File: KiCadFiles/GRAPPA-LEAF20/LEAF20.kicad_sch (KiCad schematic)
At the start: 48 parts

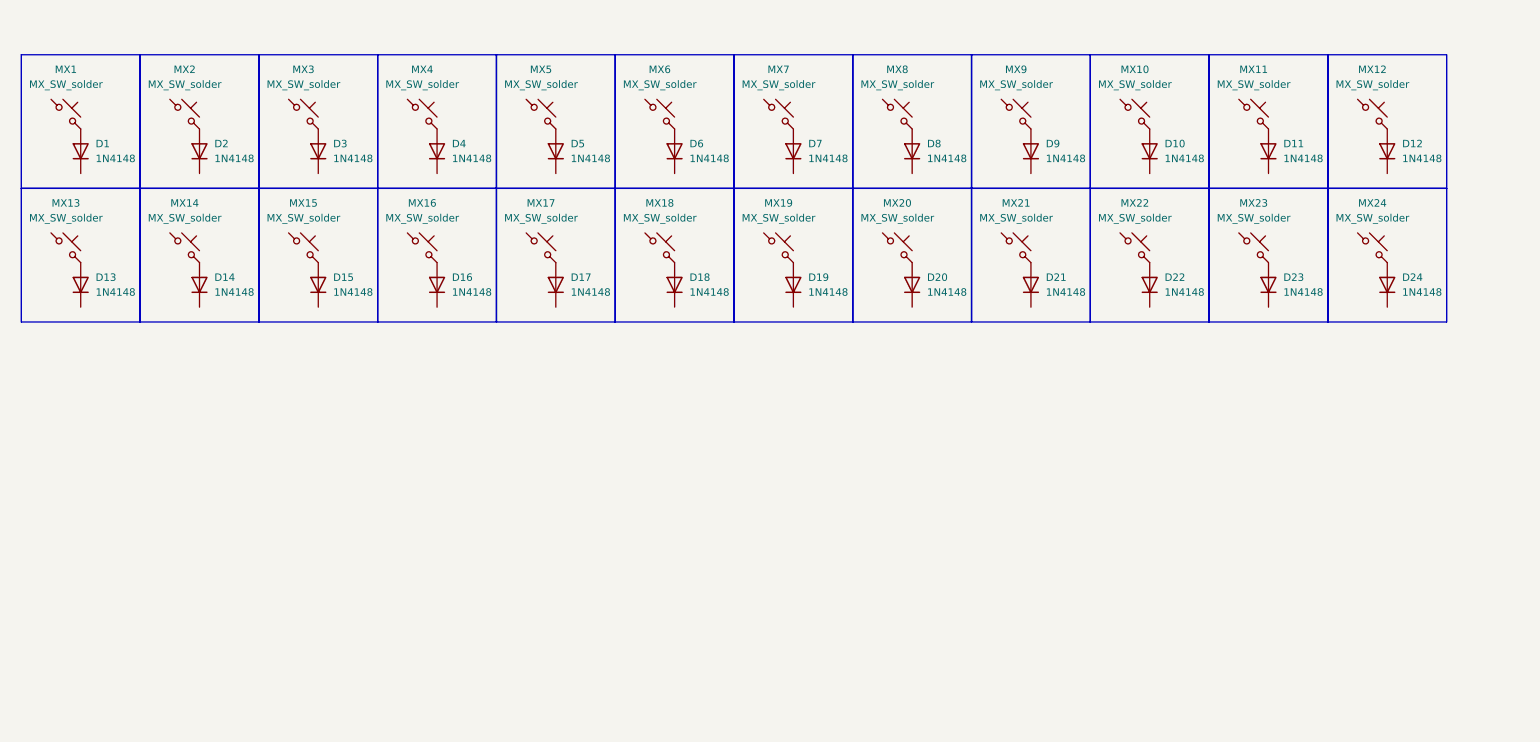
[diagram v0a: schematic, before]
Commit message: Refactor code structure for improved readability and maintainability
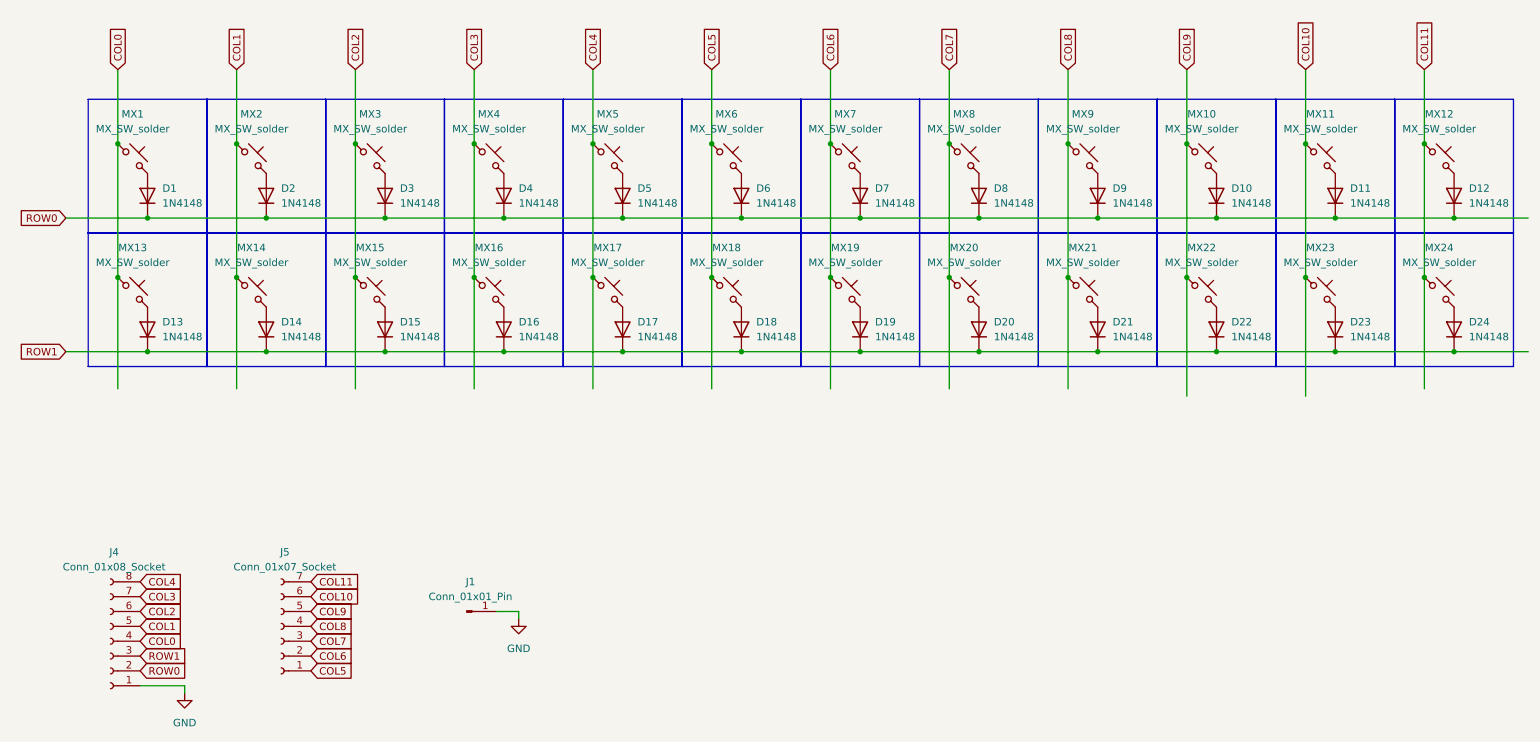
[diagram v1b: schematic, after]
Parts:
- added J1: Conn_01x01_Pin, Connector_Wire:SolderWire-0.75sqmm_1x01_D1.25mm_OD2.3mm, symbol Connector:Conn_01x01_Pin
- added J4: Conn_01x08_Socket, Connector_JST:JST_SH_SM08B-SRSS-TB_1x08-1MP_P1.00mm_Horizontal, symbol Connector:Conn_01x08_Socket
- added J5: Conn_01x07_Socket, Connector_JST:JST_SH_SM07B-SRSS-TB_1x07-1MP_P1.00mm_Horizontal, symbol Connector:Conn_01x07_Socket
- D1, D10, D11, D12, D13, D14, D15, D16, D17, D18, D19, D2, D20, D21, D22, D23, D24, D3, D4, D5, D6, D7, D8, D9: footprint Diode_SMD:D_SOD-323_HandSoldering -> My-Fi Footprints:D_SOD-123-g
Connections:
- net COL3: now reaches MX16.1
- net COL3: now also MX4.1, J4.7 (Pin_7)
- net ROW0: now reaches D12.1 (K)
- net ROW0: now also D1.1 (K), D10.1 (K), D11.1 (K), D2.1 (K), D3.1 (K), D4.1 (K), D5.1 (K), D6.1 (K), D7.1 (K), D8.1 (K), D9.1 (K), J4.2 (Pin_2)
- net ROW1: now reaches D19.1 (K)
- net ROW1: now also D13.1 (K), D14.1 (K), D15.1 (K), D16.1 (K), D17.1 (K), D18.1 (K), D20.1 (K), D21.1 (K), D22.1 (K), D23.1 (K), D24.1 (K), J4.3 (Pin_3)
- net COL2: now reaches MX3.1
- net COL2: now also MX15.1, J4.6 (Pin_6)
- net COL5: now reaches MX18.1
- net COL5: now also MX6.1, J5.1 (Pin_1)
- net COL4: now reaches MX17.1
- net COL4: now also MX5.1, J4.8 (Pin_8)
- net COL10: now reaches MX23.1
- net COL10: now also MX11.1, J5.6 (Pin_6)
- net COL11: now reaches MX12.1
- net COL11: now also MX24.1, J5.7 (Pin_7)
- net COL7: now reaches MX20.1
- net COL7: now also MX8.1, J5.3 (Pin_3)
- net COL6: now reaches MX7.1
- net COL6: now also MX19.1, J5.2 (Pin_2)
- net COL9: now reaches MX10.1
- net COL9: now also MX22.1, J5.5 (Pin_5)
- net COL0: now reaches MX13.1
- net COL0: now also MX1.1, J4.4 (Pin_4)
- net COL1: now reaches MX14.1
- net COL1: now also MX2.1, J4.5 (Pin_5)
- net COL8: now reaches MX9.1
- net COL8: now also MX21.1, J5.4 (Pin_4)
- new net GND: J1.1 (Pin_1), J4.1 (Pin_1)
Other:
- moved on the sheet: D1, D10, D11, D12, D13, D14, D15, D16, D17, D18, D19, D2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
